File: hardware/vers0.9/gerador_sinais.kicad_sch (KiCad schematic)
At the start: 13 parts, among them J1 COMUNIC, J2 JTAG, J3 Conn_01x03, J7 Fonte 5v, J8 Fonte 12V, J9 Fonte 12V, U4 74HC00, U5 74HC00, U8 74HC00, U9 74HC00

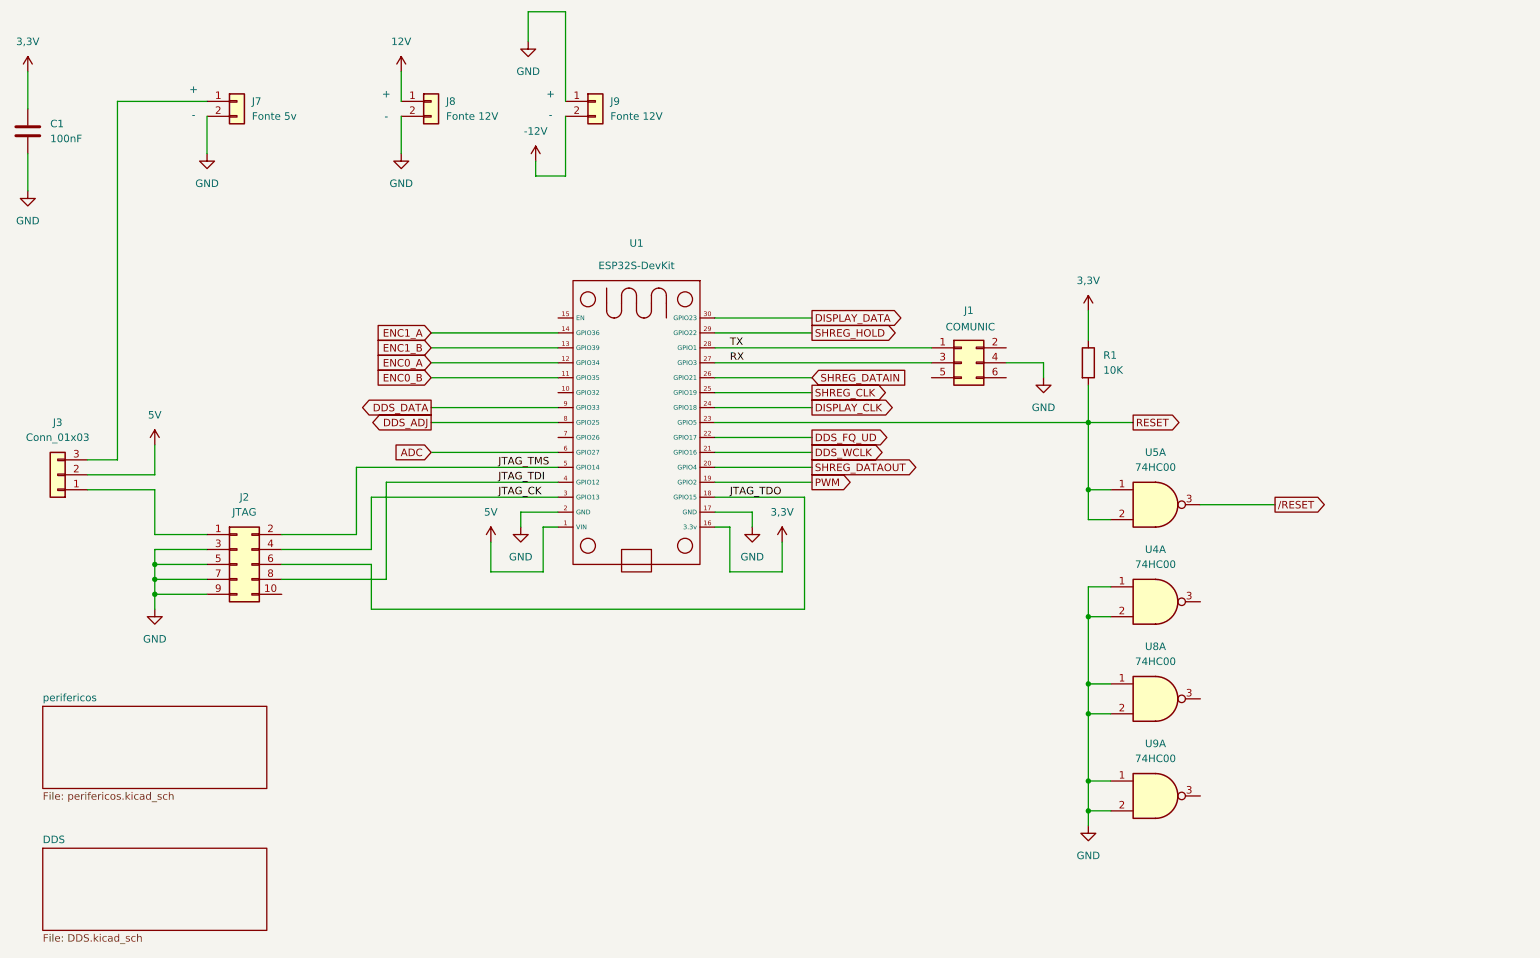
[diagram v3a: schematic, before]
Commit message: 250427-1145
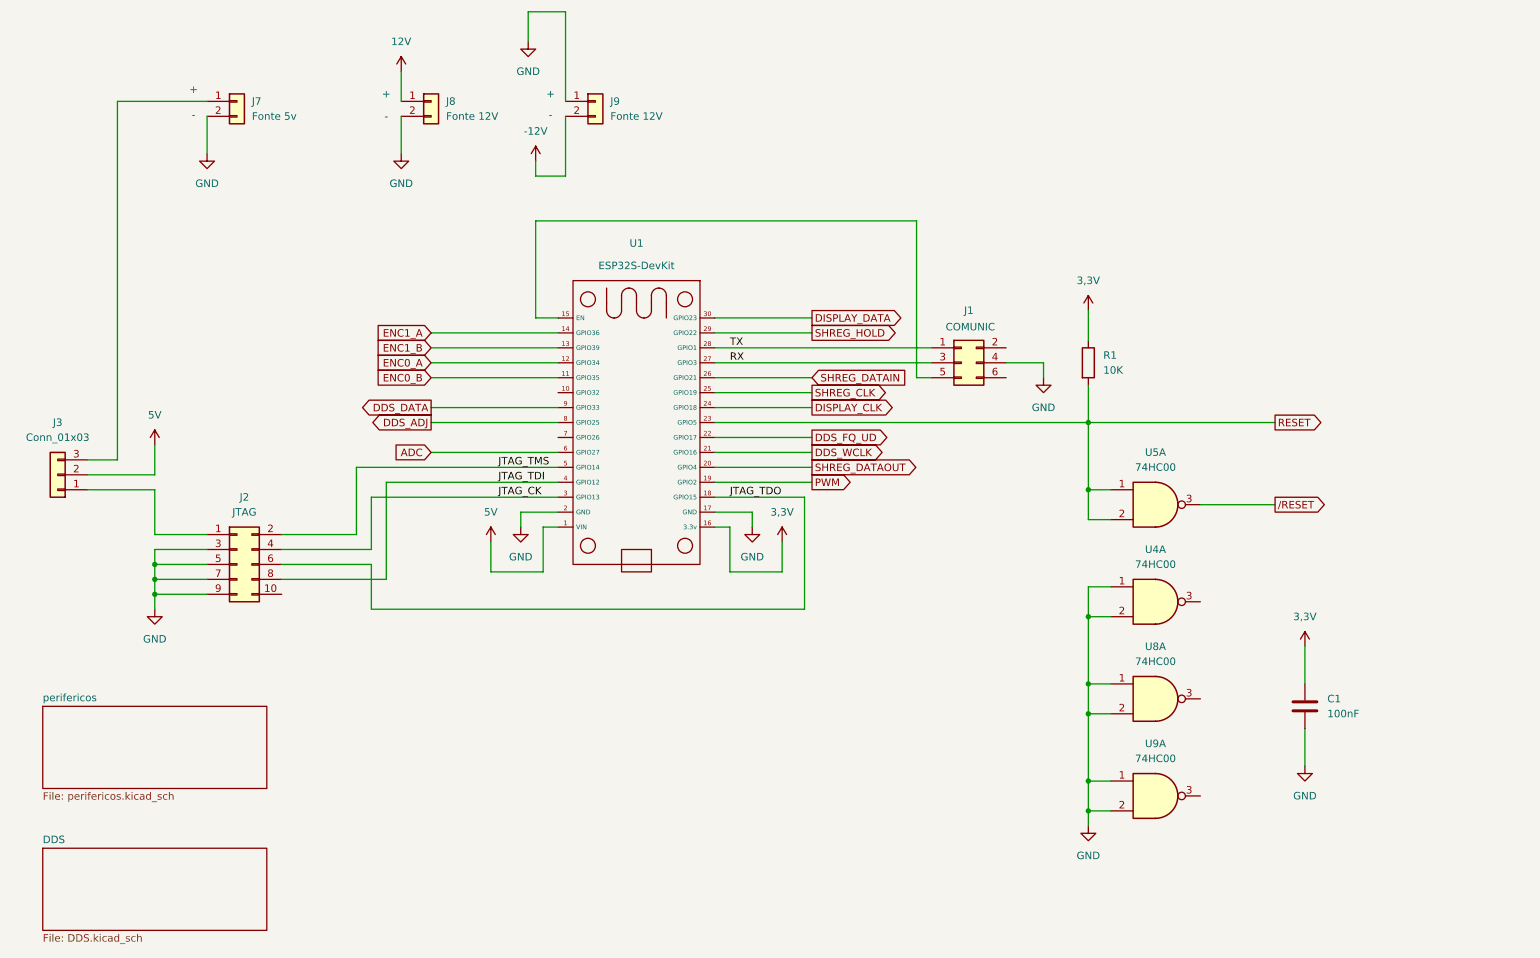
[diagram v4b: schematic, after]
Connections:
- net at J1.5 (Pin_5): now also U1.15 (EN)
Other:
- moved on the sheet: C1
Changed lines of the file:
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@@
 	(wire
 		(pts
-			(xy 203.2 88.9) (xy 210.82 88.9)
+			(xy 203.2 88.9) (xy 234.95 88.9)
 		)
 		(stroke
@@
 	(wire
 		(pts
+			(xy 173.99 81.28) (xy 173.99 54.61)
+		)
+		(stroke
+			(width 0)
+			(type default)
+		)
+	)
+	(wire
+		(pts
 			(xy 107.95 19.05) (xy 107.95 24.13)
 		)
@@
 	(wire
 		(pts
+			(xy 109.22 71.12) (xy 113.03 71.12)
+		)
+		(stroke
+			(width 0)
+			(type default)
+		)
+	)
+	(wire
+		(pts
 			(xy 86.36 29.21) (xy 86.36 34.29)
 		)
@@
 	(wire
 		(pts
+			(xy 109.22 54.61) (xy 109.22 71.12)
+		)
+		(stroke
+			(width 0)
+			(type default)
+		)
+	)
+	(wire
+		(pts
 			(xy 53.34 34.29) (xy 38.1 34.29)
 		)
@@
 	(wire
 		(pts
+			(xy 173.99 54.61) (xy 109.22 54.61)
+		)
+		(stroke
+			(width 0)
+			(type default)
+		)
+	)
+	(wire
+		(pts
 			(xy 139.7 96.52) (xy 156.21 96.52)
 		)
@@
 	(wire
 		(pts
-			(xy 22.86 43.18) (xy 22.86 49.53)
+			(xy 240.03 140.97) (xy 240.03 147.32)
 		)
 		(stroke
@@
 	(wire
 		(pts
-			(xy 22.86 29.21) (xy 22.86 35.56)
+			(xy 240.03 127) (xy 240.03 133.35)
 		)
 		(stroke
@@
 		(pts
 			(xy 203.2 69.85) (xy 203.2 74.93)
+		)
+		(stroke
+			(width 0)
+			(type default)
+		)
+	)
+	(wire
+		(pts
+			(xy 176.53 81.28) (xy 173.99 81.28)
 		)
 		(stroke
@@
 	(global_label "RESET"
 		(shape output)
-		(at 210.82 88.9 0)
+		(at 234.95 88.9 0)
 		(fields_autoplaced yes)
 		(effects
@@
 		)
 		(property "Intersheetrefs" "${INTERSHEET_REFS}"
-			(at 219.5503 88.9 0)
+			(at 243.6803 88.9 0)
 			(effects
 				(font
@@
 	(symbol
 		(lib_id "Device:C")
-		(at 22.86 39.37 0)
+		(at 240.03 137.16 0)
 		(unit 1)
 		(exclude_from_sim no)
@@
 		(fields_autoplaced yes)
 		(property "Reference" "C1"
-			(at 26.67 38.0999 0)
+			(at 243.84 135.8899 0)
 			(effects
 				(font
@@
 		)
 		(property "Value" "100nF"
-			(at 26.67 40.6399 0)
+			(at 243.84 138.4299 0)
 			(effects
 				(font
@@
 		)
 		(property "Footprint" ""
-			(at 23.8252 43.18 0)
+			(at 240.9952 140.97 0)
 			(effects
 				(font
@@
 		)
 		(property "Datasheet" "~"
-			(at 22.86 39.37 0)
+			(at 240.03 137.16 0)
 			(effects
 				(font
@@
 		)
 		(property "Description" "Unpolarized capacitor"
-			(at 22.86 39.37 0)
+			(at 240.03 137.16 0)
 			(effects
 				(font
@@
 	(symbol
 		(lib_id "power:VCC")
-		(at 22.86 29.21 0)
+		(at 240.03 127 0)
 		(unit 1)
 		(exclude_from_sim no)
@@
 		(dnp no)
 		(property "Reference" "#PWR12"
-			(at 22.86 33.02 0)
+			(at 240.03 130.81 0)
 			(effects
 				(font
@@
 		)
 		(property "Value" "3,3V"
-			(at 22.86 24.13 0)
+			(at 240.03 121.92 0)
 			(effects
 				(font
@@
 		)
 		(property "Footprint" ""
-			(at 22.86 29.21 0)
+			(at 240.03 127 0)
 			(effects
 				(font
@@
 		)
 		(property "Datasheet" ""
-			(at 22.86 29.21 0)
+			(at 240.03 127 0)
 			(effects
 				(font
@@
 		)
 		(property "Description" "Power symbol creates a global label with name \"VCC\""
-			(at 22.86 29.21 0)
+			(at 240.03 127 0)
 			(effects
 				(font
@@
 	(symbol
 		(lib_id "power:GND")
-		(at 22.86 49.53 0)
+		(at 240.03 147.32 0)
 		(unit 1)
 		(exclude_from_sim no)
@@
 		(fields_autoplaced yes)
 		(property "Reference" "#PWR11"
-			(at 22.86 55.88 0)
+			(at 240.03 153.67 0)
 			(effects
 				(font
@@
 		)
 		(property "Value" "GND"
-			(at 22.86 54.61 0)
+			(at 240.03 152.4 0)
 			(effects
 				(font
@@
 		)
 		(property "Footprint" ""
-			(at 22.86 49.53 0)
+			(at 240.03 147.32 0)
 			(effects
 				(font
@@
 		)
 		(property "Datasheet" ""
-			(at 22.86 49.53 0)
+			(at 240.03 147.32 0)
 			(effects
 				(font
@@
 		)
 		(property "Description" "Power symbol creates a global label with name \"GND\" , ground"
-			(at 22.86 49.53 0)
-			(effects
-				(font
+			(at 240.03 147.32 0)
+			(effects
+				(font

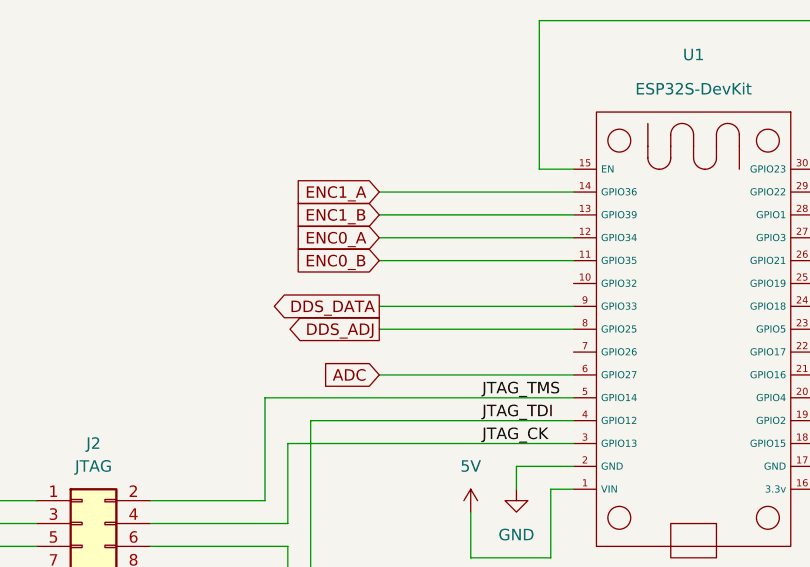
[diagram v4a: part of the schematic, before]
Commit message: 250826-1410
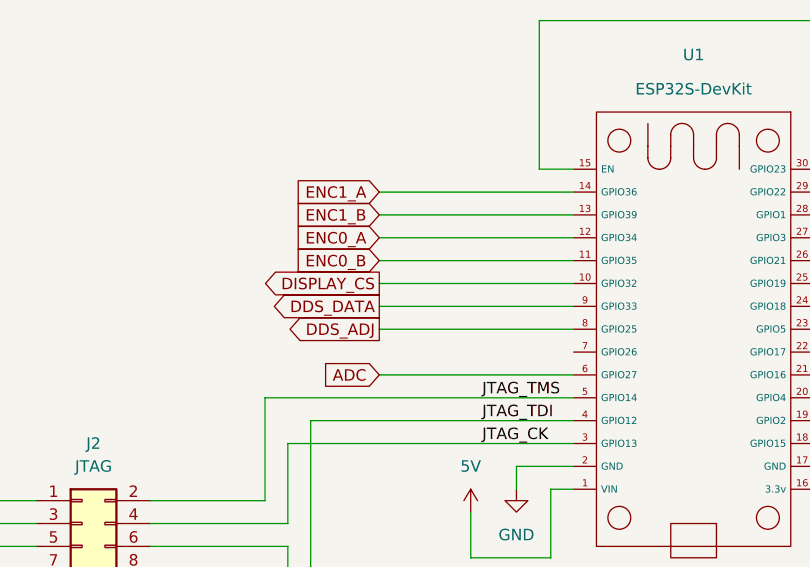
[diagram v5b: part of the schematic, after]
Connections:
- net DISPLAY_CS: now reaches U1.10 (GPIO32)
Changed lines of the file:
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@@
+	(wire
+		(pts
+			(xy 91.44 83.82) (xy 113.03 83.82)
+		)
+		(stroke
+			(width 0)
+			(type default)
+		)
+	)
 	(wire
 		(pts
@@
 				(hide yes)
 			)
+		)
+	)
+	(global_label "DISPLAY_CS"
+		(shape output)
+		(at 91.44 83.82 180)
+		(fields_autoplaced yes)
+		(effects
+			(font
+				(size 1.27 1.27)
+			)
+			(justify right)
+		)
+		(property "Intersheetrefs" "${INTERSHEET_REFS}"
+			(at 77.4481 83.82 0)
+			(effects
+				(font
+					(size 1.27 1.27)
+				)
+				(justify right)
+				(hide yes)
+			)

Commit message: 250827-1625
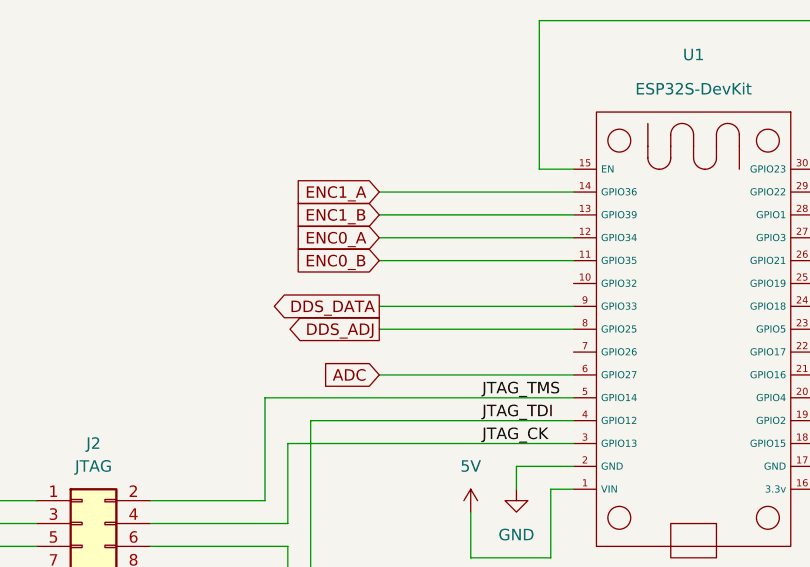
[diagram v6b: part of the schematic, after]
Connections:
- net DISPLAY_CS: no longer names the net of U1.10 (GPIO32)
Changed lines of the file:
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@@
-	(wire
-		(pts
-			(xy 91.44 83.82) (xy 113.03 83.82)
-		)
-		(stroke
-			(width 0)
-			(type default)
-		)
-	)
 	(wire
 		(pts
@@
 				(hide yes)
 			)
-		)
-	)
-	(global_label "DISPLAY_CS"
-		(shape output)
-		(at 91.44 83.82 180)
-		(fields_autoplaced yes)
-		(effects
-			(font
-				(size 1.27 1.27)
-			)
-			(justify right)
-		)
-		(property "Intersheetrefs" "${INTERSHEET_REFS}"
-			(at 77.4481 83.82 0)
-			(effects
-				(font
-					(size 1.27 1.27)
-				)
-				(justify right)
-				(hide yes)
-			)
